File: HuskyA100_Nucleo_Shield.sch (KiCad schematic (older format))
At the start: 18 parts, among them CN10 HEADER_17x2, CN7 HEADER_10x2, CN8 HEADER_8x2, CN9 HEADER_15x2, J1 Conn_01x03, J2 Conn_01x03, J3 Conn_01x04, J4 Conn_01x04

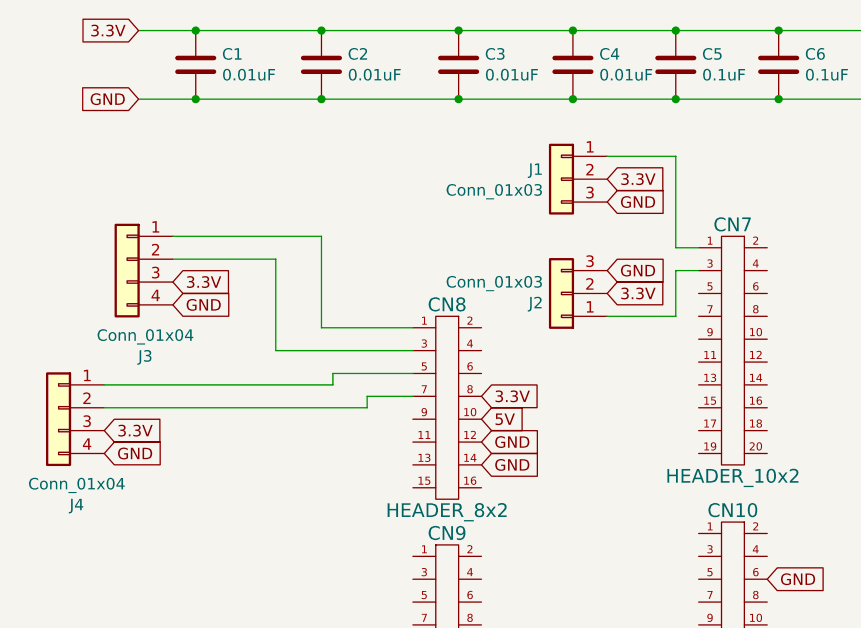
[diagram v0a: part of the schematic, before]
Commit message: added a title, miscellaneous fixes changes
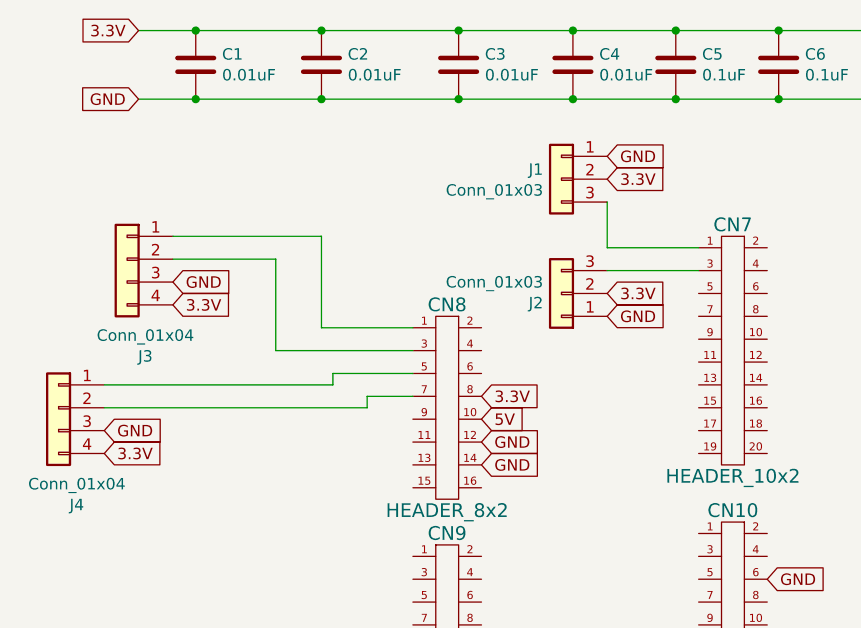
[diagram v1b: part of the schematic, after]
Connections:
- net 3.3V: now also J3.4 (Pin_4), J4.4 (Pin_4); no longer J3.3 (Pin_3), J4.3 (Pin_3)
- net GND: now also J1.1 (Pin_1), J2.1 (Pin_1), J3.3 (Pin_3), J4.3 (Pin_3); no longer J1.3 (Pin_3), J2.3 (Pin_3), J3.4 (Pin_4), J4.4 (Pin_4)
- net at CN7.1: now also J1.3 (Pin_3); no longer J1.1 (Pin_1)
- net at CN7.3: now also J2.3 (Pin_3); no longer J2.1 (Pin_1)
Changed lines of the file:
@@
 Text GLabel 4450 3800 2    50   Input ~ 0
 3.3V
+Text GLabel 2800 4050 2    50   Input ~ 0
+3.3V
+Text GLabel 3100 3400 2    50   Input ~ 0
+3.3V
+Text GLabel 5000 3450 2    50   Input ~ 0
+GND
+Text GLabel 5000 3350 2    50   Input ~ 0
+3.3V
+Text GLabel 3100 3300 2    50   Input ~ 0
+GND
 Text GLabel 2800 3950 2    50   Input ~ 0
-3.3V
-Text GLabel 3100 3300 2    50   Input ~ 0
-3.3V
-Text GLabel 5000 3250 2    50   Input ~ 0
-GND
-Text GLabel 5000 3350 2    50   Input ~ 0
-3.3V
-Text GLabel 3100 3400 2    50   Input ~ 0
-GND
-Text GLabel 2800 4050 2    50   Input ~ 0
 GND
 Text GLabel 4150 5000 0    50   Input ~ 0
@@
 Text GLabel 5000 2850 2    50   Input ~ 0
 3.3V
-Text GLabel 5000 2950 2    50   Input ~ 0
-GND
-Wire Wire Line
-	5000 2750 5300 2750
-Wire Wire Line
-	5300 2750 5300 3150
-Wire Wire Line
-	5300 3150 5400 3150
-Wire Wire Line
-	5000 3450 5300 3450
-Wire Wire Line
-	5300 3450 5300 3250
-Wire Wire Line
-	5300 3250 5400 3250
+Text GLabel 5000 2750 2    50   Input ~ 0
+GND
 Wire Wire Line
 	2950 2200 3200 2200
@@
 Text GLabel 5700 4600 2    50   Input ~ 0
 GND
+Wire Wire Line
+	5000 3150 5000 2950
+Wire Wire Line
+	5000 3150 5400 3150
+Wire Wire Line
+	5000 3250 5400 3250
 $EndSCHEMATC
